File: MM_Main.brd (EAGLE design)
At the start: 74 x 87.2 mm, 81 parts, among them IC1 ULN2003AD, IC2 TB6612FNG, IC4 LD117ADT50TR, IC5 MCP1825, Q1 TEFT4300, Q2 TEFT4300, Q3 TEFT4300, Q4 TEFT4300, Q5 TEFT4300, Q6 TEFT4300, Q8 8MHz

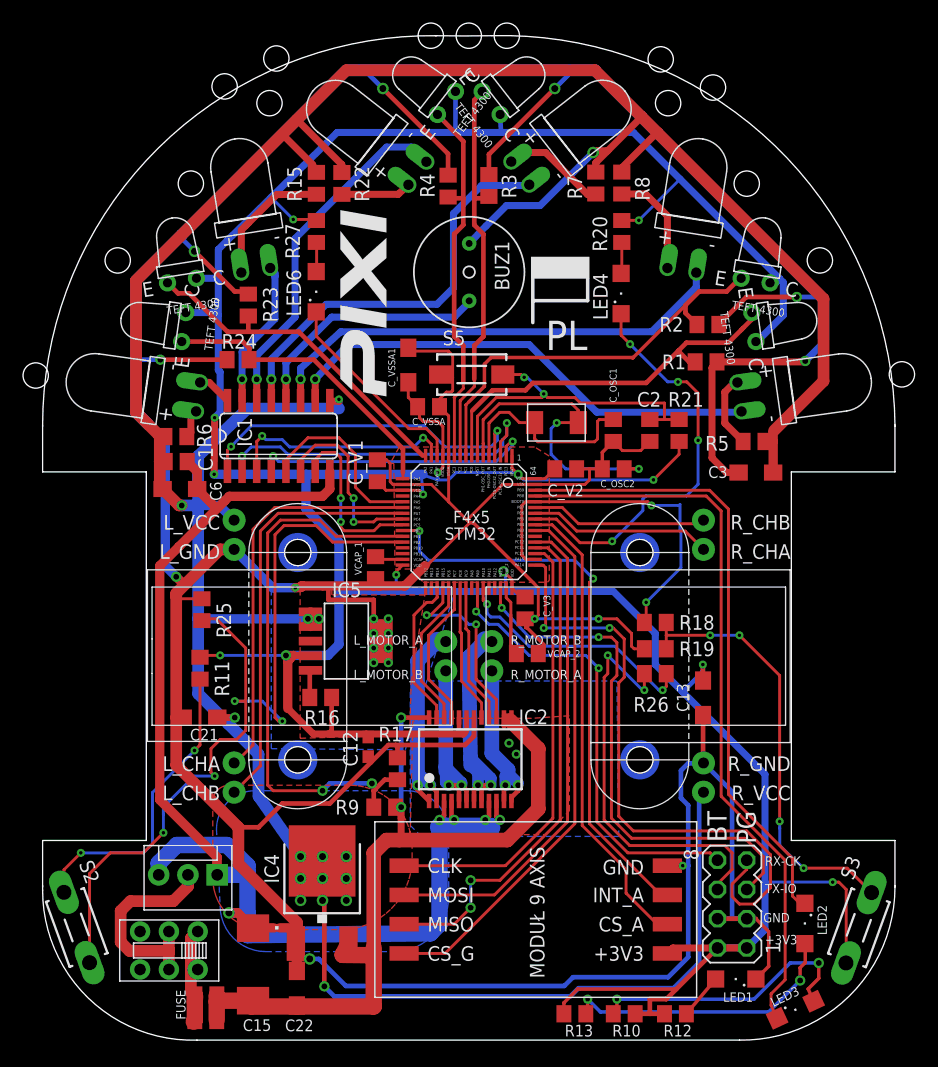
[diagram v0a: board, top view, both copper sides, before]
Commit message: drobne poprawki, chyba koniec :P
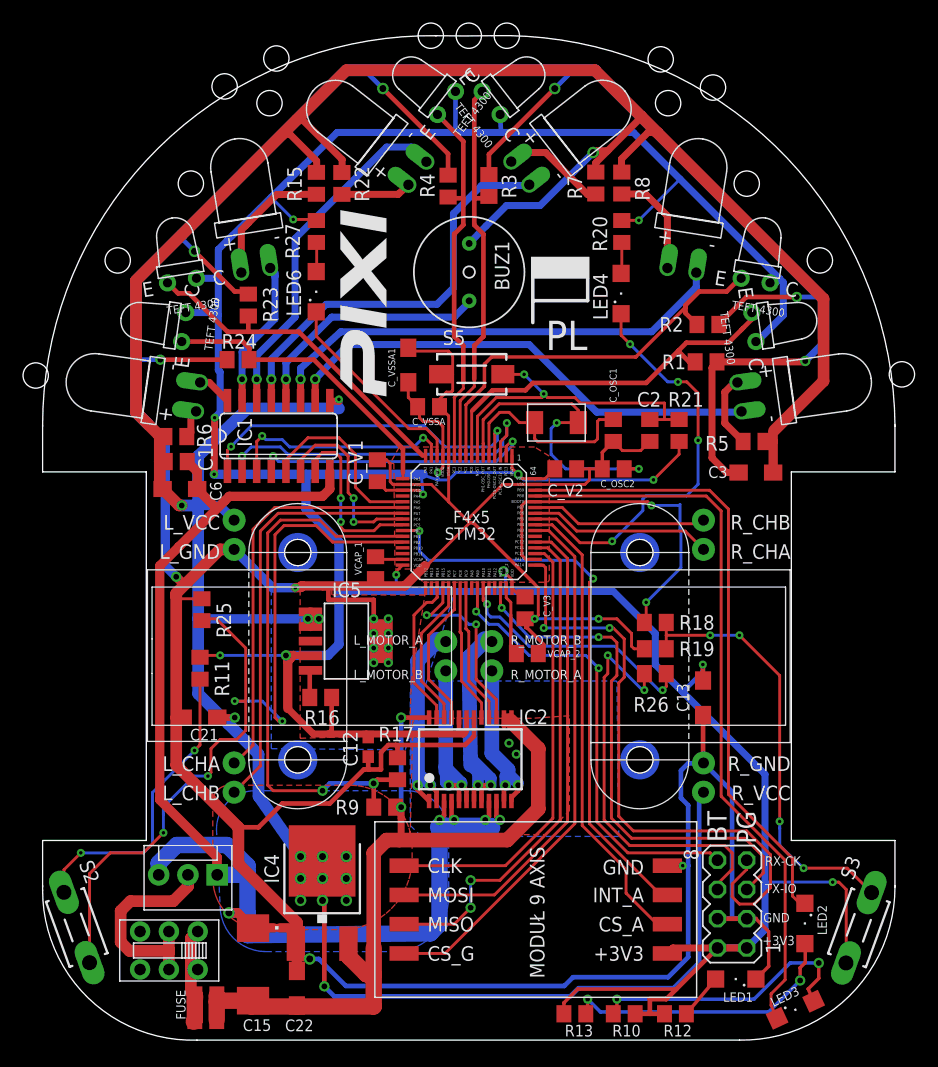
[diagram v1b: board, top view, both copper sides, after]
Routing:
- net +5V: track 296.5 -> 298.1 mm
- net GND: track 465.0 -> 466.4 mm
- net BTN: track 76.3 -> 75.7 mm
